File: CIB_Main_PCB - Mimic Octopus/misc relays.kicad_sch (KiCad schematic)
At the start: 7 parts, among them U3 ULN2803A, U4 MCP23017_SO, U5 ULN2803A, U6 ULN2803A, U7 MCP23017_SO

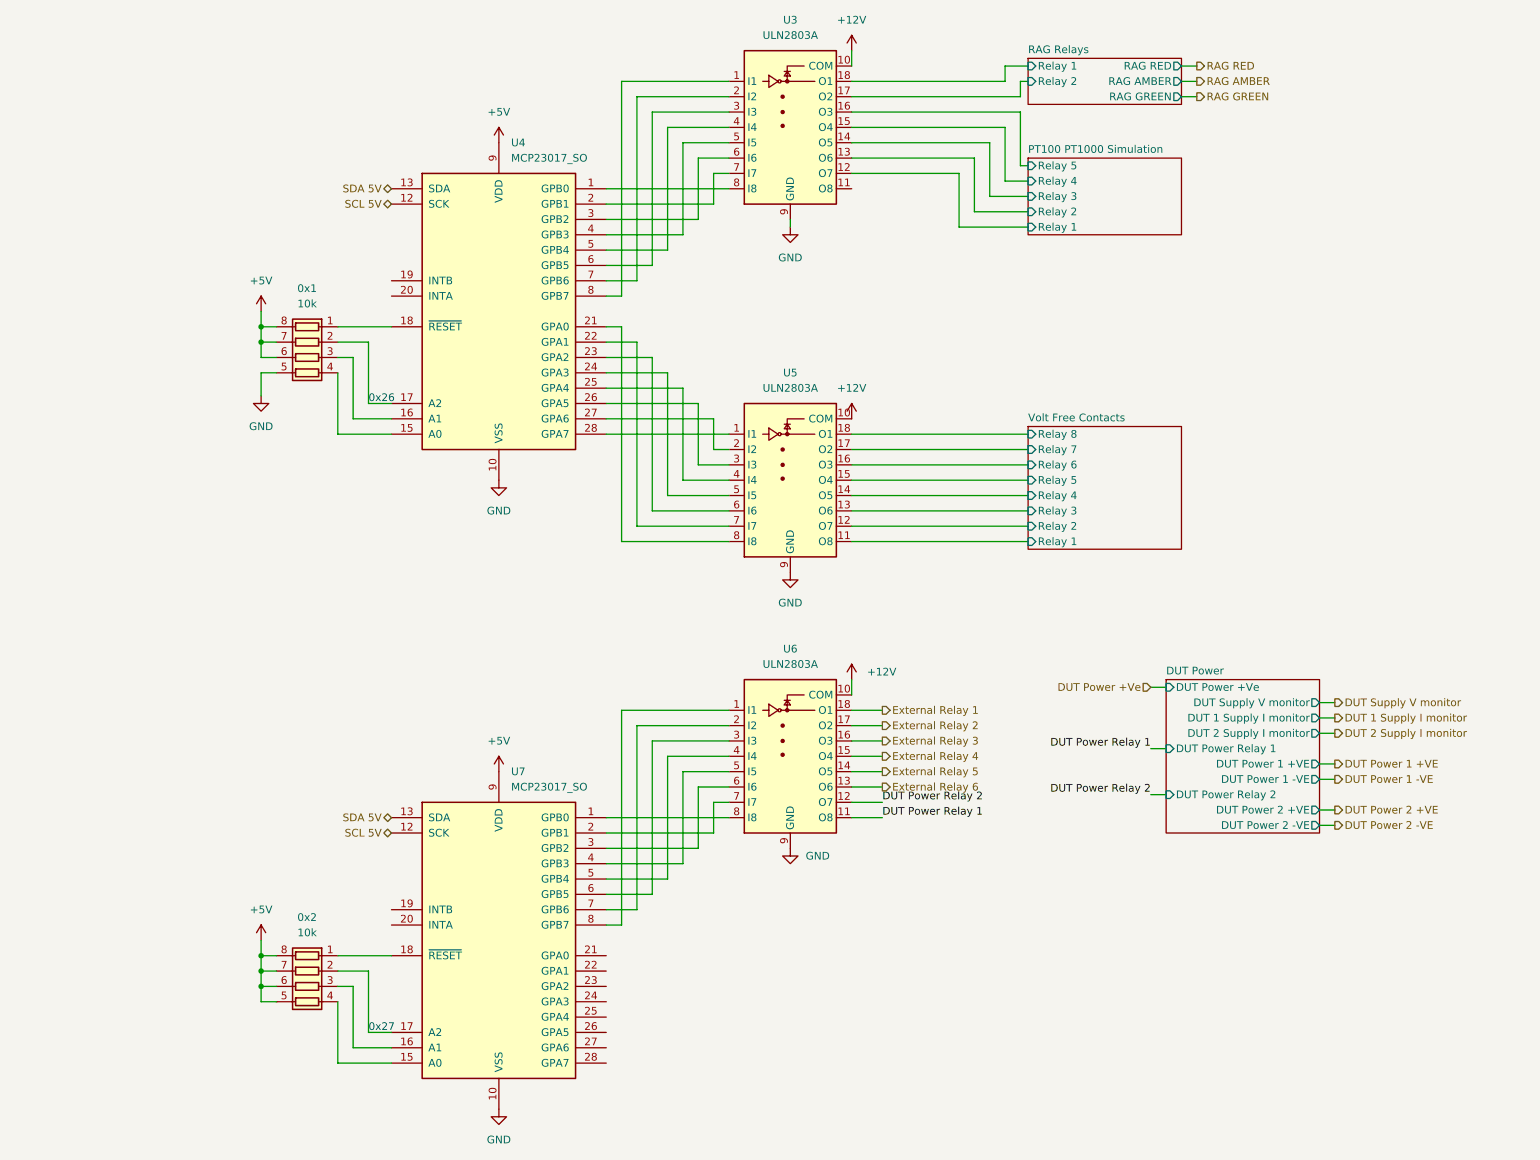
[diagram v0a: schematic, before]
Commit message: V0.1 PCB to be sent out
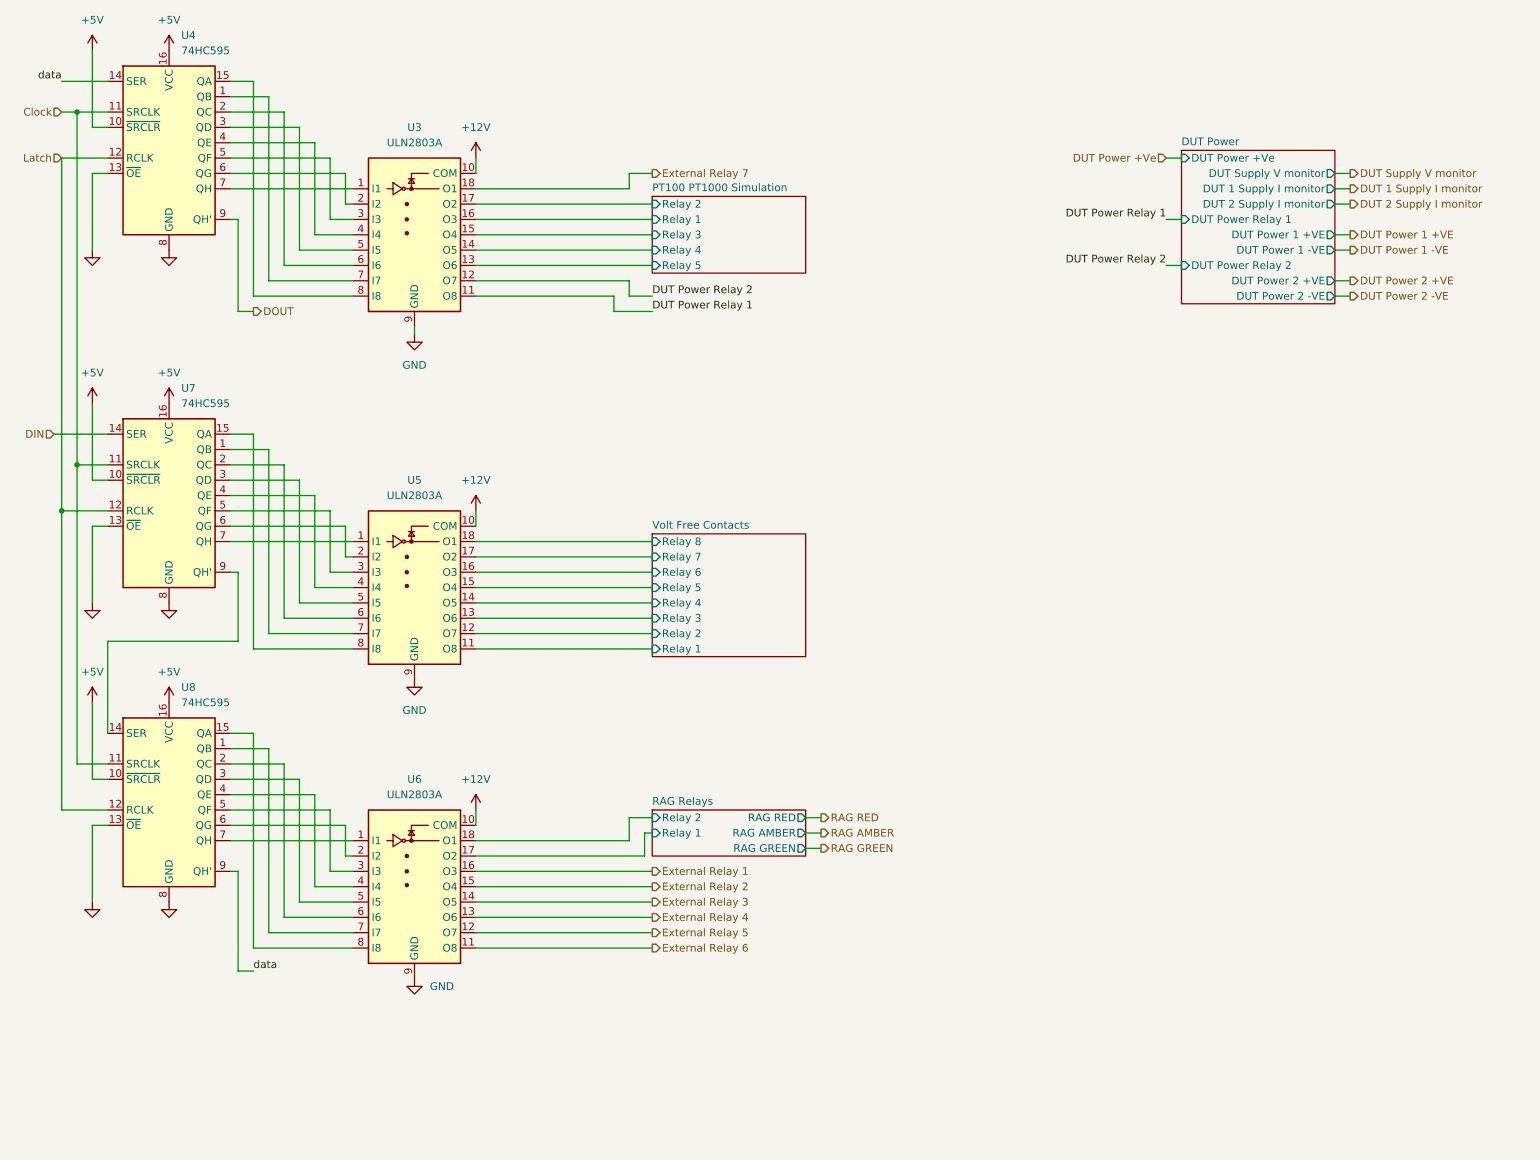
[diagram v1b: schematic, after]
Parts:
- removed 0x1, 0x2: 10k, Resistor_SMD:R_Array_Convex_4x1206, symbol Device:R_Pack04
- removed U4, U7: MCP23017_SO, Package_SO:SOIC-28W_7.5x17.9mm_P1.27mm, symbol Interface_Expansion:MCP23017_SO
- added U4, U7, U8: 74HC595, Package_DIP:DIP-16_W7.62mm_LongPads, symbol 74xx:74HC595
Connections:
- net +5V: now also U4.10 (~{SRCLR}), U4.16 (VCC), U7.10 (~{SRCLR}), U7.16 (VCC), U8.10 (~{SRCLR}), U8.16 (VCC)
- net DUT Power Relay 1: now also U3.11 (O8); no longer U6.11 (O8)
- net DUT Power Relay 2: now also U3.12 (O7); no longer U6.12 (O7)
- net External Relay 1: now also U6.16 (O3); no longer U6.18 (O1)
- net External Relay 2: now also U6.15 (O4); no longer U6.17 (O2)
- net External Relay 3: now also U6.14 (O5); no longer U6.16 (O3)
- net External Relay 4: now also U6.13 (O6); no longer U6.15 (O4)
- net External Relay 5: now also U6.12 (O7); no longer U6.14 (O5)
- net External Relay 6: now also U6.11 (O8); no longer U6.13 (O6)
- net GND: now also U4.13 (~{OE}), U4.8 (GND), U7.13 (~{OE}), U7.8 (GND), U8.13 (~{OE}), U8.8 (GND)
- net PT100 PT1000 Simulation/Relay 1: now also U3.16 (O3); no longer U3.12 (O7)
- net PT100 PT1000 Simulation/Relay 2: now also U3.17 (O2); no longer U3.13 (O6)
- net PT100 PT1000 Simulation/Relay 3: now also U3.15 (O4); no longer U3.14 (O5)
- net PT100 PT1000 Simulation/Relay 4: now also U3.14 (O5); no longer U3.15 (O4)
- net PT100 PT1000 Simulation/Relay 5: now also U3.13 (O6); no longer U3.16 (O3)
- net RAG Relays/Relay 1: now also U6.17 (O2); no longer U3.18 (O1)
- net RAG Relays/Relay 2: now also U6.18 (O1); no longer U3.17 (O2)
- net at U5.1 (I1): now also U7.7 (QH)
- net at U5.2 (I2): now also U7.6 (QG)
- net at U5.3 (I3): now also U7.5 (QF)
- net at U5.4 (I4): now also U7.4 (QE)
- net at U5.5 (I5): now also U7.3 (QD)
- net at U5.6 (I6): now also U7.2 (QC)
- net at U5.7 (I7): now also U7.1 (QB)
- net at U5.8 (I8): now also U7.15 (QA)
- net at U6.8 (I8): now also U8.15 (QA)
- net at U6.7 (I7): now also U8.1 (QB)
- net at U6.6 (I6): now also U8.2 (QC)
- net at U6.5 (I5): now also U8.3 (QD)
- net at U6.4 (I4): now also U8.4 (QE)
- net at U6.3 (I3): now also U8.5 (QF)
- net at U6.2 (I2): now also U8.6 (QG)
- net at U6.1 (I1): now also U8.7 (QH)
- net at U3.1 (I1): now also U4.7 (QH)
- net at U3.2 (I2): now also U4.6 (QG)
- net at U3.3 (I3): now also U4.5 (QF)
- net at U3.4 (I4): now also U4.4 (QE)
- net at U3.5 (I5): now also U4.3 (QD)
- net at U3.6 (I6): now also U4.2 (QC)
- net at U3.7 (I7): now also U4.1 (QB)
- net at U3.8 (I8): now also U4.15 (QA)
- new net: U7.9 (QH'), U8.14 (SER)
- new net Clock: U4.11 (SRCLK), U7.11 (SRCLK), U8.11 (SRCLK)
- new net DIN: U7.14 (SER)
- new net DOUT: U4.9 (QH')
- new net External Relay 7: U3.18 (O1)
- new net Latch: U4.12 (RCLK), U7.12 (RCLK), U8.12 (RCLK)
- new net data: U4.14 (SER), U8.9 (QH')
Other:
- note removed: "0x26"
- note removed: "0x27"
- moved on the sheet: U3, U5, U6

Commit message: BoM
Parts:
- U3, U5, U6: Height (none) -> 5; Mouser # (none) -> 511-ULN2803A; Mouser Part Number 511-ULN2803A -> (none)
- U4, U7, U8: Height (none) -> 5
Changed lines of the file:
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@@
+      (effects (font (size 1.27 1.27)) hide)
+    )
+    (property "Manufacturer" "STMicroelectronics" (id 7) (at 85.09 106.68 0)
+      (effects (font (size 1.27 1.27)) hide)
+    )
+    (property "Manufacturer #" "ULN2803A" (id 5) (at 85.09 106.68 0)
       (effects (font (size 1.27 1.27)) hide)
     )
@@
       (effects (font (size 1.27 1.27)) hide)
     )
-    (property "Manufacturer #" "ULN2803A" (id 5) (at 85.09 106.68 0)
-      (effects (font (size 1.27 1.27)) hide)
-    )
-    (property "Manufacturere" "" (id 6) (at 85.09 106.68 0)
-      (effects (font (size 1.27 1.27)) hide)
-    )
-    (property "Manufacturer" "STMicroelectronics" (id 7) (at 85.09 106.68 0)
-      (effects (font (size 1.27 1.27)) hide)
-    )
-    (property "Mouser #" "" (id 8) (at 85.09 106.68 0)
-      (effects (font (size 1.27 1.27)) hide)
-    )
-    (property "Mouser Part Number" "511-ULN2803A" (id 9) (at 85.09 106.68 0)
+    (property "Mouser #" "511-ULN2803A" (id 8) (at 85.09 106.68 0)
+      (effects (font (size 1.27 1.27)) hide)
+    )
+    (property "Mouser Part Number" "" (id 9) (at 85.09 106.68 0)
+      (effects (font (size 1.27 1.27)) hide)
+    )
+    (property "Height" "5" (id 10) (at 85.09 106.68 0)
       (effects (font (size 1.27 1.27)) hide)
     )
@@
       (effects (font (size 1.27 1.27)) hide)
     )
+    (property "Manufacturer" "STMicroelectronics" (id 7) (at 85.09 48.26 0)
+      (effects (font (size 1.27 1.27)) hide)
+    )
+    (property "Manufacturer #" "ULN2803A" (id 5) (at 85.09 48.26 0)
+      (effects (font (size 1.27 1.27)) hide)
+    )
     (property "DigiKey #" "497-2356-5-ND" (id 4) (at 85.09 48.26 0)
       (effects (font (size 1.27 1.27)) hide)
     )
-    (property "Manufacturer #" "ULN2803A" (id 5) (at 85.09 48.26 0)
-      (effects (font (size 1.27 1.27)) hide)
-    )
-    (property "Manufacturere" "" (id 6) (at 85.09 48.26 0)
-      (effects (font (size 1.27 1.27)) hide)
-    )
-    (property "Manufacturer" "STMicroelectronics" (id 7) (at 85.09 48.26 0)
-      (effects (font (size 1.27 1.27)) hide)
-    )
-    (property "Mouser #" "" (id 8) (at 85.09 48.26 0)
-      (effects (font (size 1.27 1.27)) hide)
-    )
-    (property "Mouser Part Number" "511-ULN2803A" (id 9) (at 85.09 48.26 0)
+    (property "Mouser #" "511-ULN2803A" (id 8) (at 85.09 48.26 0)
+      (effects (font (size 1.27 1.27)) hide)
+    )
+    (property "Mouser Part Number" "" (id 9) (at 85.09 48.26 0)
+      (effects (font (size 1.27 1.27)) hide)
+    )
+    (property "Height" "5" (id 10) (at 85.09 48.26 0)
       (effects (font (size 1.27 1.27)) hide)
     )
@@
       (effects (font (size 1.27 1.27)) hide)
     )
+    (property "Height" "5" (id 4) (at 44.45 93.98 0)
+      (effects (font (size 1.27 1.27)) hide)
+    )
     (pin "1")
     (pin "10")
@@
       (effects (font (size 1.27 1.27)) hide)
     )
+    (property "Height" "5" (id 4) (at 44.45 35.56 0)
+      (effects (font (size 1.27 1.27)) hide)
+    )
     (pin "1")
     (pin "10")
@@
     )
     (property "Datasheet" "http://www.ti.com/lit/ds/symlink/sn74hc595.pdf" (id 3) (at 44.45 143.51 0)
+      (effects (font (size 1.27 1.27)) hide)
+    )
+    (property "Height" "5" (id 4) (at 44.45 143.51 0)
       (effects (font (size 1.27 1.27)) hide)
     )
@@
       (effects (font (size 1.27 1.27)) hide)
     )
+    (property "Manufacturer" "STMicroelectronics" (id 7) (at 85.09 156.21 0)
+      (effects (font (size 1.27 1.27)) hide)
+    )
+    (property "Manufacturer #" "ULN2803A" (id 5) (at 85.09 156.21 0)
+      (effects (font (size 1.27 1.27)) hide)
+    )
     (property "DigiKey #" "497-2356-5-ND" (id 4) (at 85.09 156.21 0)
       (effects (font (size 1.27 1.27)) hide)
     )
-    (property "Manufacturer #" "ULN2803A" (id 5) (at 85.09 156.21 0)
-      (effects (font (size 1.27 1.27)) hide)
-    )
-    (property "Manufacturere" "" (id 6) (at 85.09 156.21 0)
-      (effects (font (size 1.27 1.27)) hide)
-    )
-    (property "Manufacturer" "STMicroelectronics" (id 7) (at 85.09 156.21 0)
-      (effects (font (size 1.27 1.27)) hide)
-    )
-    (property "Mouser #" "" (id 8) (at 85.09 156.21 0)
-      (effects (font (size 1.27 1.27)) hide)
-    )
-    (property "Mouser Part Number" "511-ULN2803A" (id 9) (at 85.09 156.21 0)
-      (effects (font (size 1.27 1.27)) hide)
-    )
+    (property "Mouser #" "511-ULN2803A" (id 8) (at 85.09 156.21 0)
+      (effects (font (size 1.27 1.27)) hide)
+    )
+    (property "Mouser Part Number" "" (id 9) (at 85.09 156.21 0)
+      (effects (font (size 1.27 1.27)) hide)
+    )
+    (property "Height" "5" (id 10) (at 85.09 156.21 0)
+      (effects (font (size 1.27 1.27)) hide)
+    )
